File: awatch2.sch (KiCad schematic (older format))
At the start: 0 parts

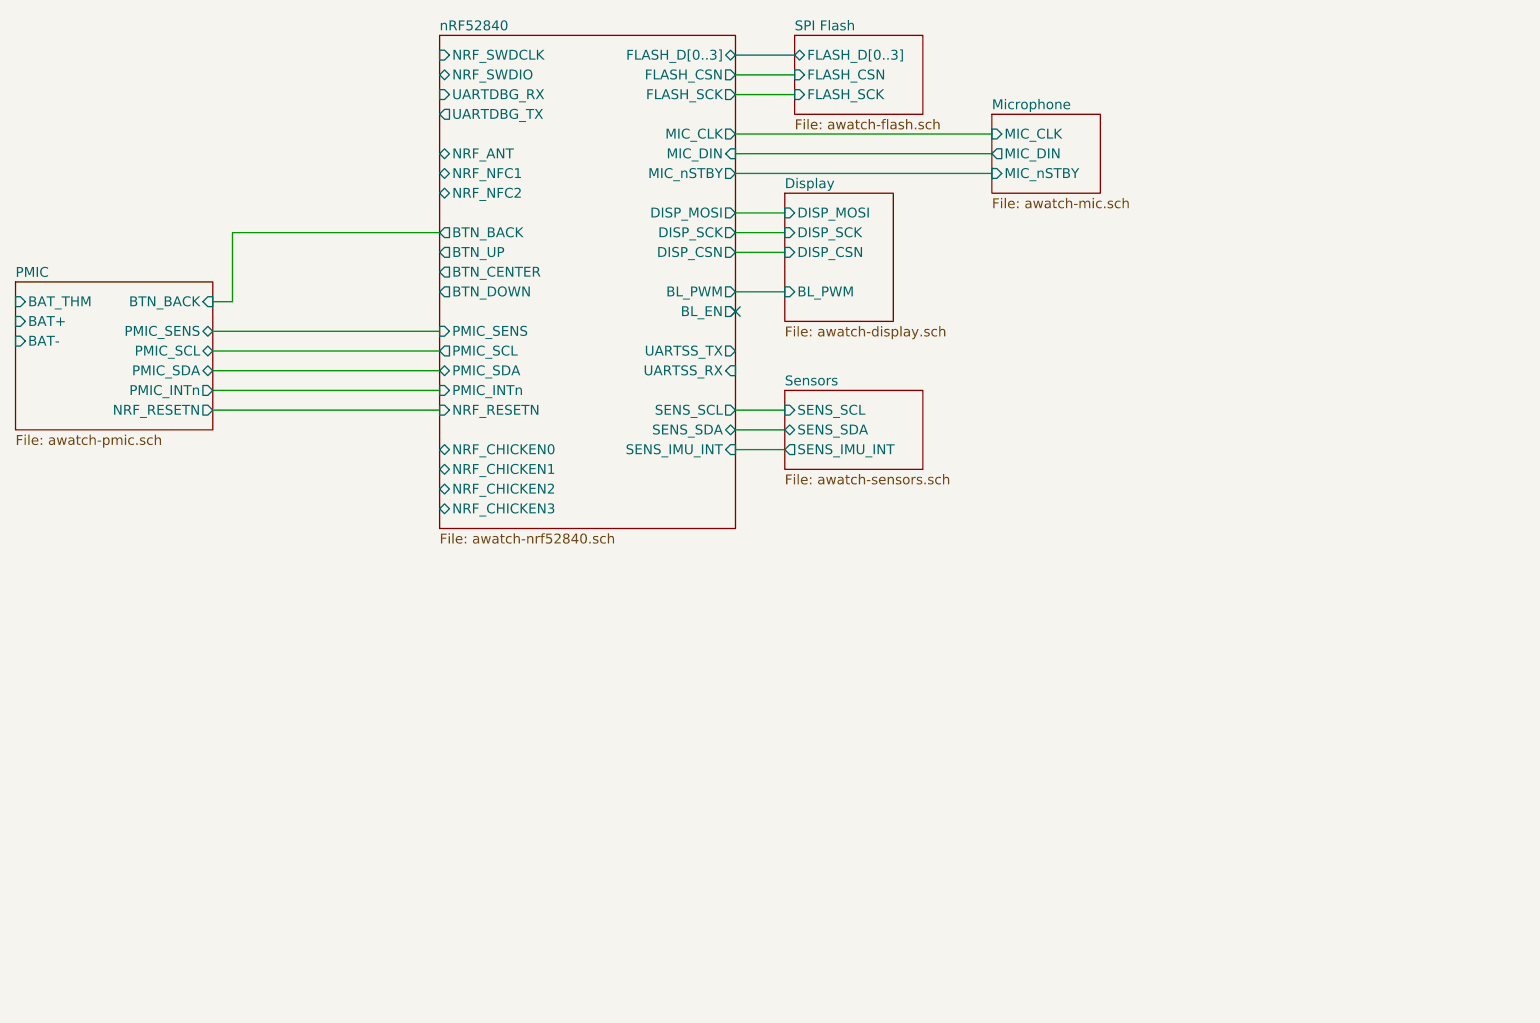
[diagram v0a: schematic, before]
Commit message: add FTDI
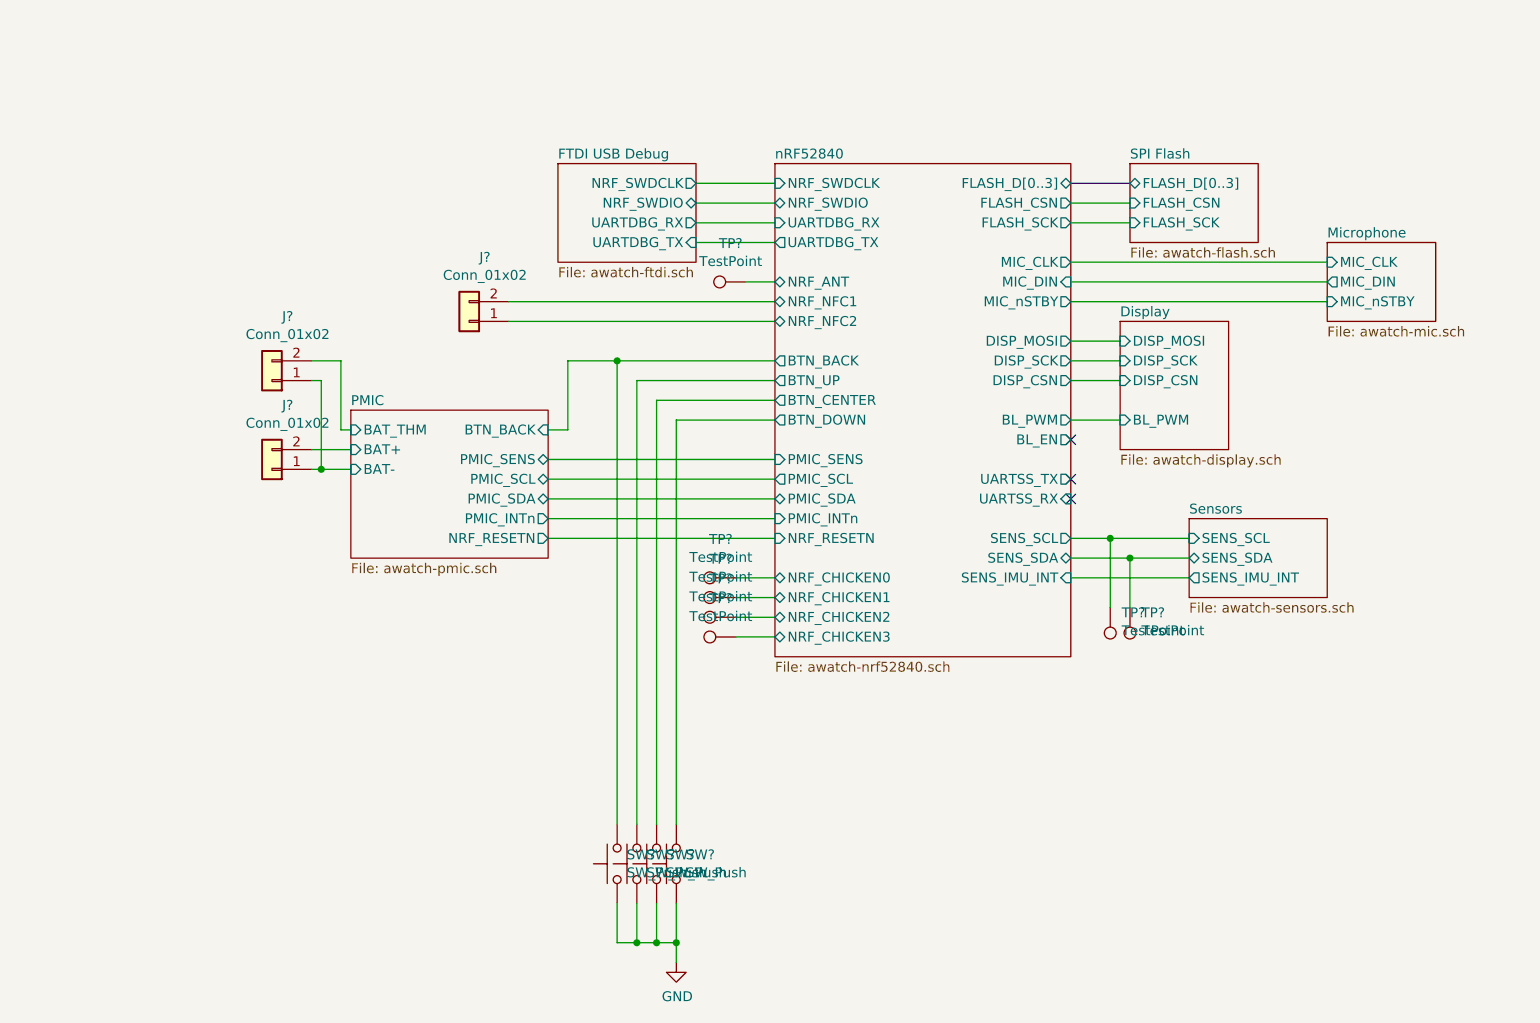
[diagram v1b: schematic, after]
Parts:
- added J? (x3): Conn_01x02, symbol Connector_Generic:Conn_01x02
- added SW? (x4): SW_Push, symbol Switch:SW_Push
- added TP? (x7): TestPoint, symbol Connector:TestPoint
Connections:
- net PMIC/BAT+: now also J?.2 (Pin_2)
- net PMIC/BAT-: now also J?.1 (Pin_1), J?.1 (Pin_1)
- net PMIC/BAT_THM: now also J?.2 (Pin_2)
- net PMIC/BTN_BACK: now also SW?.2
- net Sensors/SENS_SCL: now also TP?.1
- net Sensors/SENS_SDA: now also TP?.1
- net nRF52840/BTN_CENTER: now also SW?.2
- net nRF52840/BTN_DOWN: now also SW?.2
- net nRF52840/BTN_UP: now also SW?.2
- net nRF52840/NRF_ANT: now also TP?.1
- net nRF52840/NRF_CHICKEN0: now also TP?.1
- net nRF52840/NRF_CHICKEN1: now also TP?.1
- net nRF52840/NRF_CHICKEN2: now also TP?.1
- net nRF52840/NRF_CHICKEN3: now also TP?.1
- net nRF52840/NRF_NFC1: now also J?.2 (Pin_2)
- net nRF52840/NRF_NFC2: now also J?.1 (Pin_1)
- new net GND: SW?.1, SW?.1, SW?.1, SW?.1
- no-connect marks 1 -> 3
